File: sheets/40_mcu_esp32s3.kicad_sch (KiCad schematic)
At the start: 18 parts, among them J401 USB4105-GF-A, J402 UART0, SW401 RESET, SW402 BOOT, U401 ESP32-S3-WROOM-1-N8R2, U402 USBLC6-2SC6

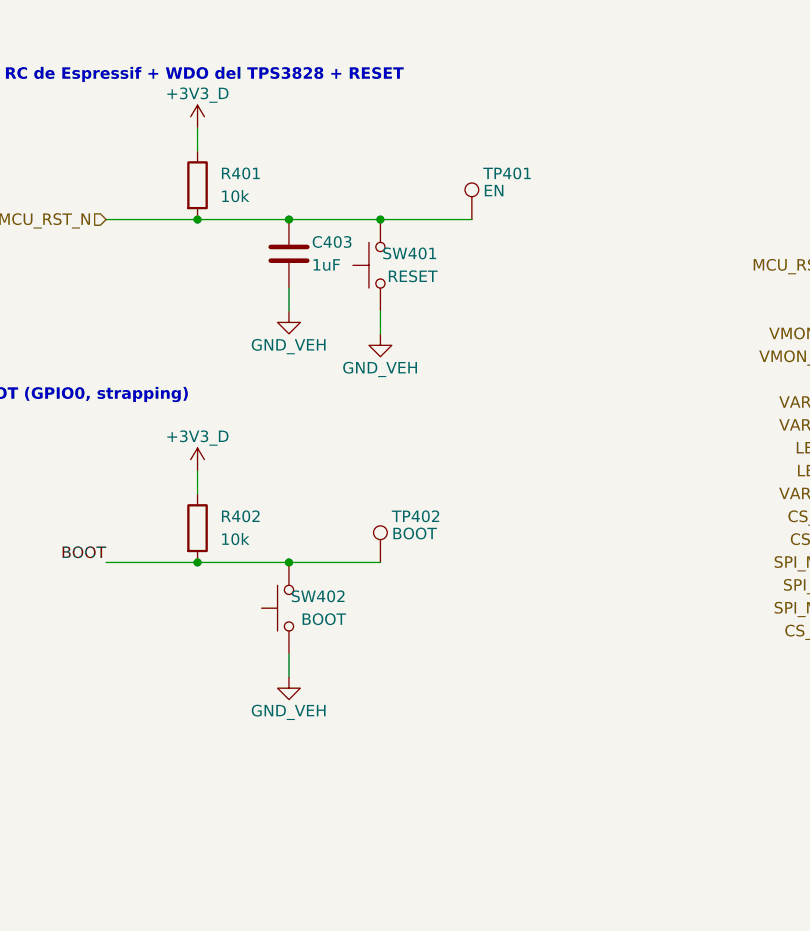
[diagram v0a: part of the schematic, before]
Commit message: update pcb layout
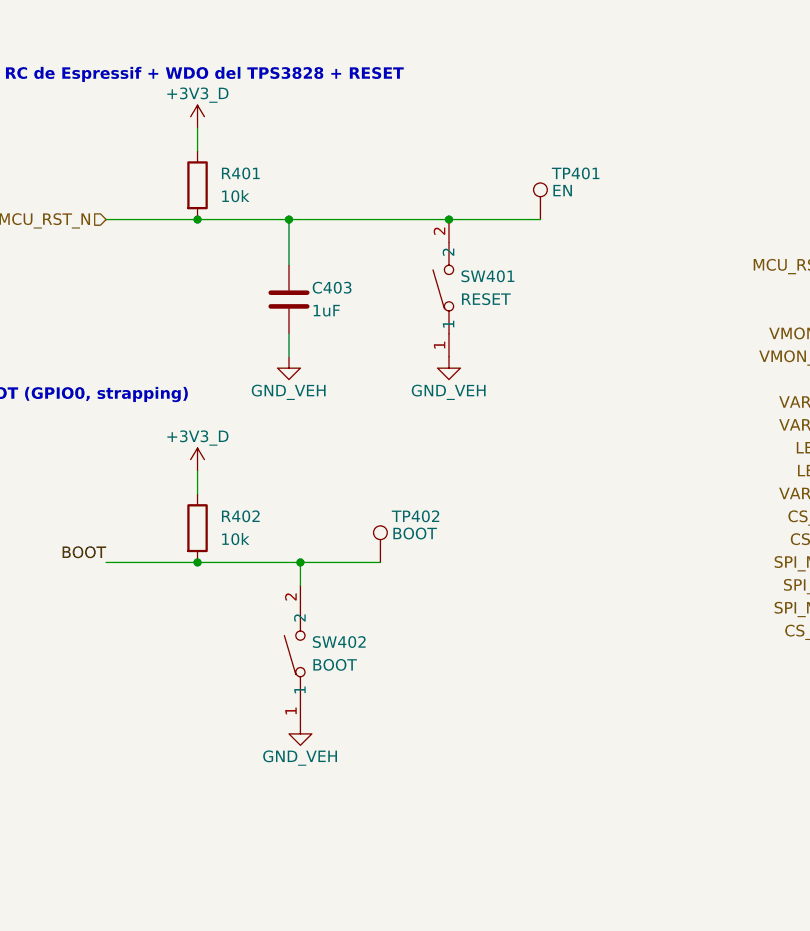
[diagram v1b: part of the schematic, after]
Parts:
- removed SW401: RESET, Button_Switch_THT:SW_PUSH_6mm, symbol Switch:SW_Push
- removed SW402: BOOT, Button_Switch_THT:SW_PUSH_6mm, symbol Switch:SW_Push
- added SW401: RESET, easyeda2kicad:SW-SMD_L3.9-W3.0-P4.45, symbol easyeda2kicad:TS-1088-AR02016
- added SW402: BOOT, easyeda2kicad:SW-SMD_L3.9-W3.0-P4.45, symbol easyeda2kicad:TS-1088-AR02016
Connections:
- net BOOT: now also SW402.2
- net GND_VEH: now also SW401.1, SW402.1
- net MCU_RST_N: now also SW401.2
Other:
- moved on the sheet: C403, TP401
